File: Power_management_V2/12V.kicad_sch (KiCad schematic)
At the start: 29 parts, among them U5 SIC43x

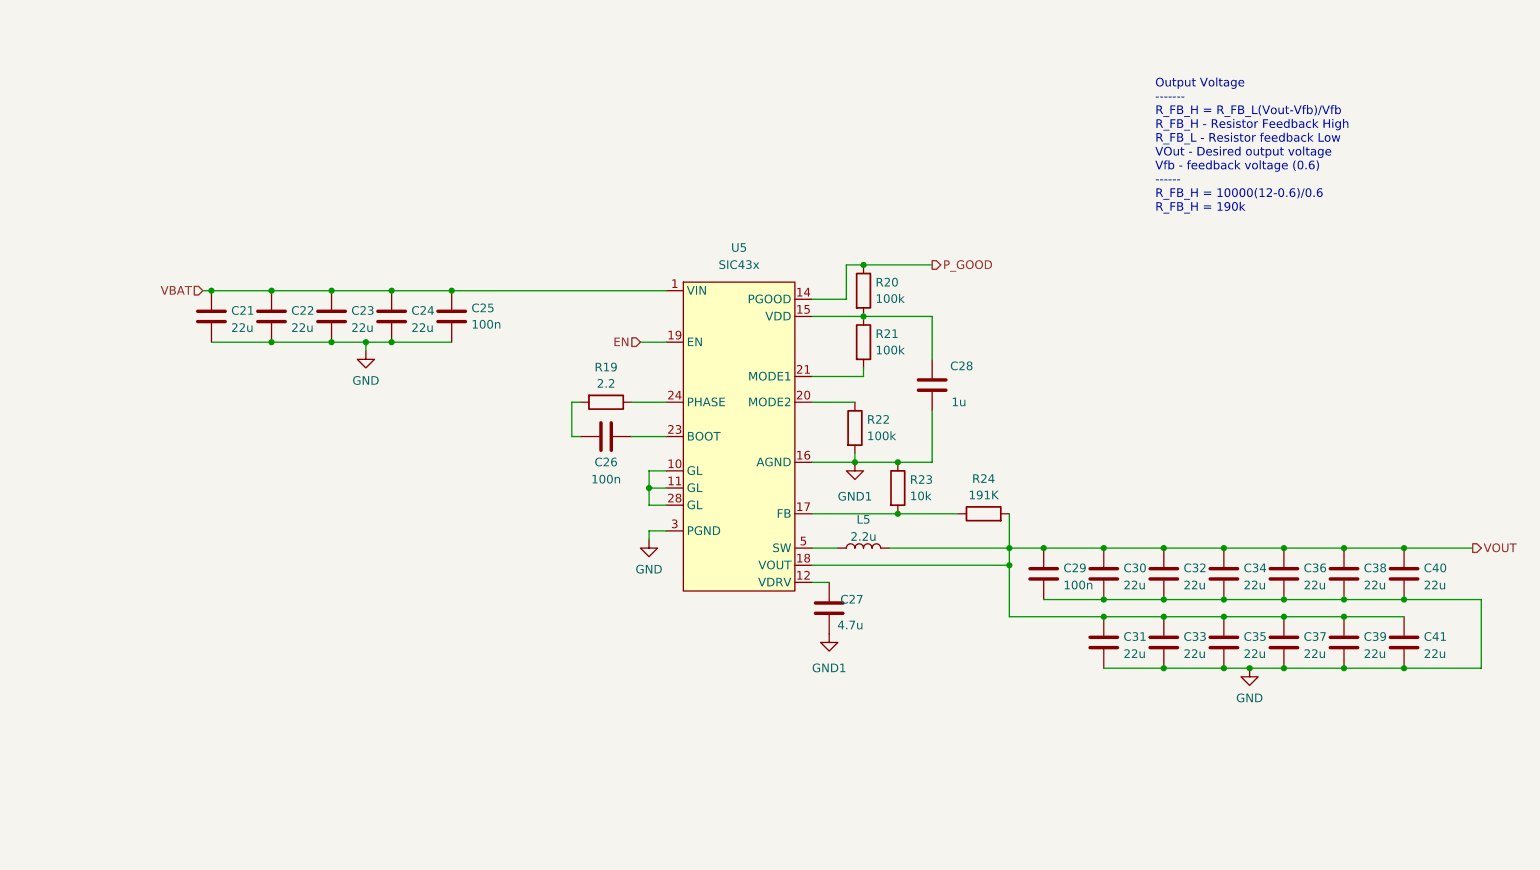
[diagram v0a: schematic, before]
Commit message: Hoan thanh SCH mach Power
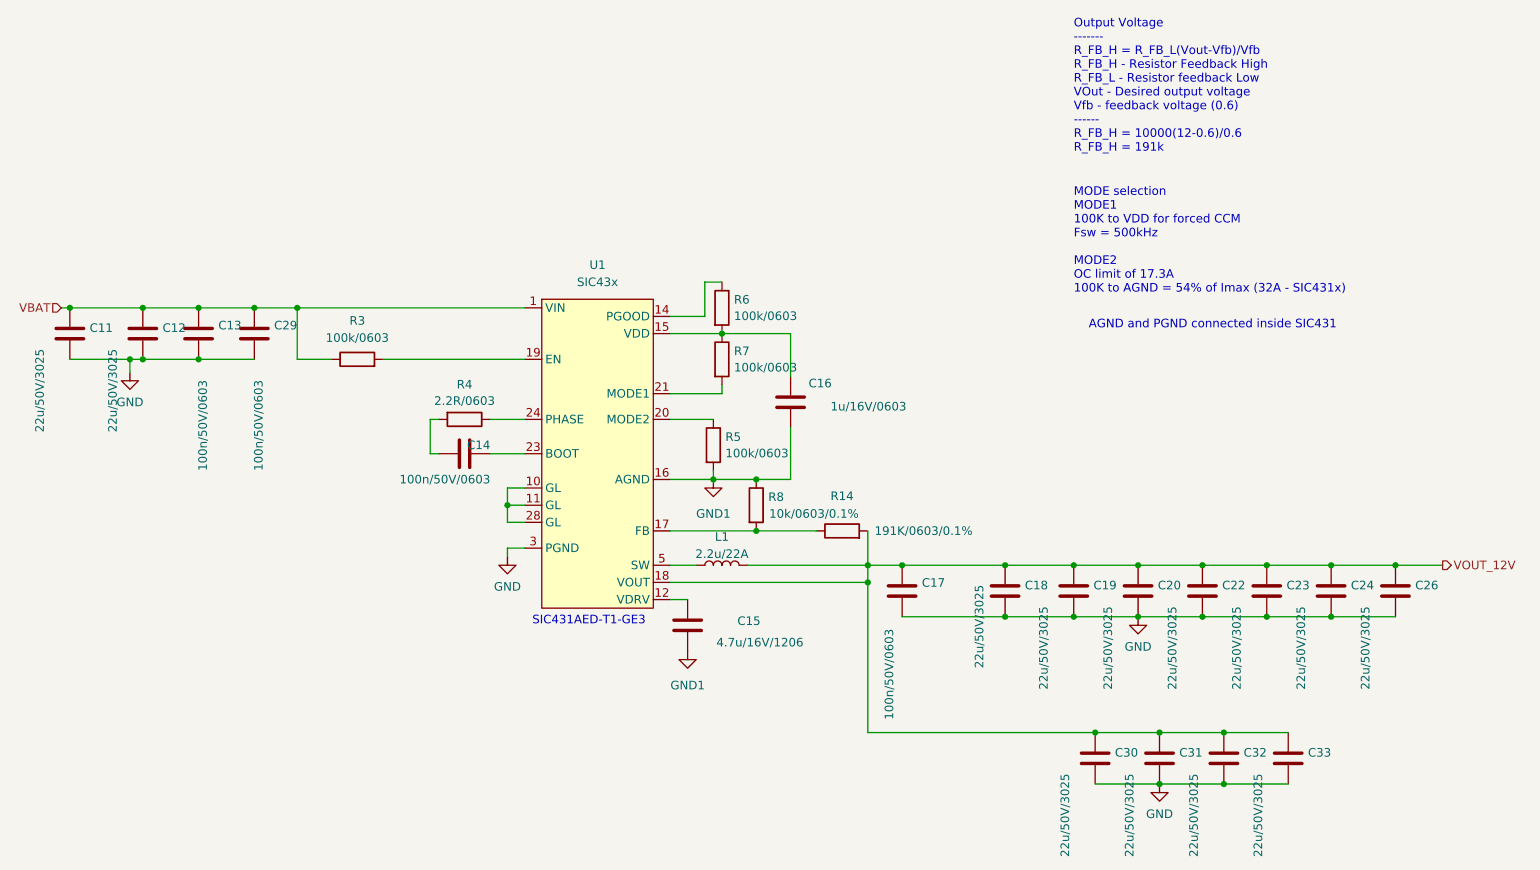
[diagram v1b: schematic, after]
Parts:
- removed C21: 22u, Library:C_CER_7.5x6.3, symbol Device:C
- removed C25: 100n, Library:C_0603_1608Metric, symbol Device:C
- removed C27: 4.7u, Library:C_1206_3216Metric, symbol Device:C
- removed C28: 1u, Library:C_0603_1608Metric, symbol Device:C
- removed C34, C35, C36, C37, C38, C39, C40, C41: 22u, Library:C_1210_3225Metric, symbol Device:C
- removed L5: 2.2u, Library:L_Vishay_IHLP-6767, symbol Device:L
- removed R19: 2.2, Library:R_0603_1608Metric, symbol Device:R
- removed R20, R21, R22: 100k, Library:R_0603_1608Metric, symbol Device:R
- removed R23: 10k, Library:R_0603_1608Metric, symbol Device:R
- removed U5: SIC43x, Library:SIC43x, symbol RM_Converter_DCDC:SIC43x
- added C11, C12, C18, C19, C20: 22u/50V/3025, Library:C_CER_7.5x6.3, symbol Device:C
- added C13, C14, C17: 100n/50V/0603, Library:C_0603_1608Metric, symbol Device:C
- added C15: 4.7u/16V/1206, Library:C_1206_3216Metric, symbol Device:C
- added C16: 1u/16V/0603, Library:C_0603_1608Metric, symbol Device:C
- added L1: 2.2u/22A, symbol Device:L
- added R3, R5, R6, R7: 100k/0603, Library:R_0603_1608Metric, symbol Device:R
- added R4: 2.2R/0603, Library:R_0603_1608Metric, symbol Device:R
- added R8: 10k/0603/0.1%, Library:R_0603_1608Metric, symbol Device:R
- added U1: SIC43x, Library:SIC43x, symbol RM_Converter_DCDC:SIC43x
- C22, C23, C24: value 22u -> 22u/50V/3025
- C26: value 100n -> 22u/50V/3025; footprint Library:C_0603_1608Metric -> Library:C_CER_7.5x6.3; Coefficient X7R -> X79; Digikey 587-1243-1-ND -> 445-174338-1-ND; Manufacturer Taiyo Yuden -> United Chemi-Con; Part UMK107B7104KA-T -> KTS500B226M76N0T00; Tolerance 10% -> 20
- C29: value 100n -> 100n/50V/0603
- C30, C31, C32, C33: value 22u -> 22u/50V/3025; footprint Library:C_1210_3225Metric -> Library:C_CER_7.5x6.3; Coefficient X7R -> X79; Digikey 1276-3392-1-ND -> 445-174338-1-ND; Manufacturer Samsung -> United Chemi-Con; Part CL32B226KAJNNNE -> KTS500B226M76N0T00; Tolerance 10% -> 20; Voltage 25 -> 50
- R14: renamed from R24; value 191K -> 191K/0603/0.1%; footprint Library:R_0603_1608Metric -> DipTek PSU library:R_0603_1608Metric; symbol Device:R -> DipTek PSU library:R
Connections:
- net GND: now also C26.2, C29.1, C11.2, C12.2, C13.1, C17.1, C18.2, C19.2, C20.2, U1.13 (PGND), U1.27 (PGND), U1.3 (PGND), U1.4 (PGND); no longer C29.2
- net GND1: now also C15.2, C16.2, R5.2, R8.1, U1.16 (AGND), U1.25 (AGND)
- net VBAT: now also C29.2, C11.1, C12.1, C13.2, R3.1, U1.1 (VIN), U1.2 (VIN), U1.22 (VIN), U1.26 (VIN); no longer C22.1, C23.1, C24.1
- net at R14.1: now also R8.2, U1.17 (FB)
- net VOUT_12V: now reaches C26.1
- net VOUT_12V: now also C22.1, C23.1, C24.1, C30.1, C31.1, C32.1, C33.1, R14.2, C17.2, C18.1, C19.1, C20.1, L1.2, U1.18 (VOUT)
- removed net VOUT: C29.1, C30.1, C31.1, C32.1, C33.1, R14.2
- new net: C16.1, R6.2, R7.1, U1.15 (VDD)
- new net: R5.1, U1.20 (MODE2)
- new net: R6.1, U1.14 (PGOOD)
- new net: R3.2, U1.19 (EN)
- new net: C14.1, U1.23 (BOOT)
- new net: C14.2, R4.2
- new net: R7.2, U1.21 (MODE1)
- new net: L1.1, U1.5 (SW), U1.6 (SW), U1.7 (SW), U1.8 (SW), U1.9 (SW)
- new net: R4.1, U1.24 (PHASE)
- new net: U1.10 (GL), U1.11 (GL), U1.28 (GL)
- new net: C15.1, U1.12 (VDRV)
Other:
- note added: "AGND and PGND connected inside SIC431"
- note added: "MODE selection MODE1 100K to VDD for forced CCM Fsw = 500kHz MODE2 OC limit of 17.3A 100K to AGND = 54% of Imax (32A - SIC431x)"
- note added: "Output Voltage ------- R_FB_H = R_FB_L(Vout-Vfb)/Vfb R_FB_H - Resistor Feedback High R_FB_L - Resistor feedback Low VOut - Desired output voltage Vfb - feedback voltage (0.6) ------ R_FB_H = 10000(12-0.6)/0.6 R_FB_H = 191k"
- note added: "SIC431AED-T1-GE3"
- note removed: "Output Voltage ------- R_FB_H = R_FB_L(Vout-Vfb)/Vfb R_FB_H - Resistor Feedback High R_FB_L - Resistor feedback Low VOut - Desired output voltage Vfb - feedback voltage (0.6) ------ R_FB_H = 10000(12-0.6)/0.6 R_FB_H = 190k"
- moved on the sheet: R14
